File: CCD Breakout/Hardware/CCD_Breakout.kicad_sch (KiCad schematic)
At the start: 6 parts, among them U1 ILX511

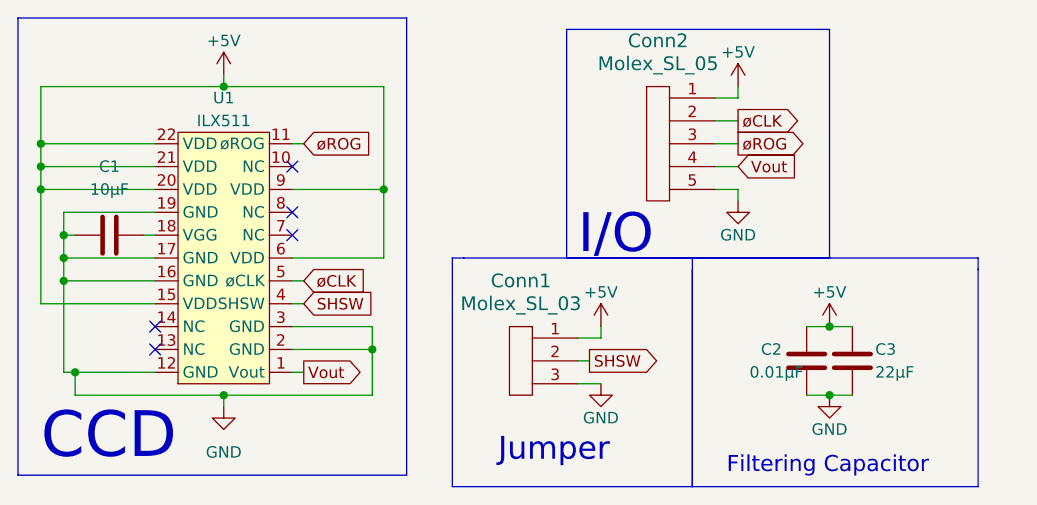
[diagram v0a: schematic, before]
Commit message: misc schematic review changes
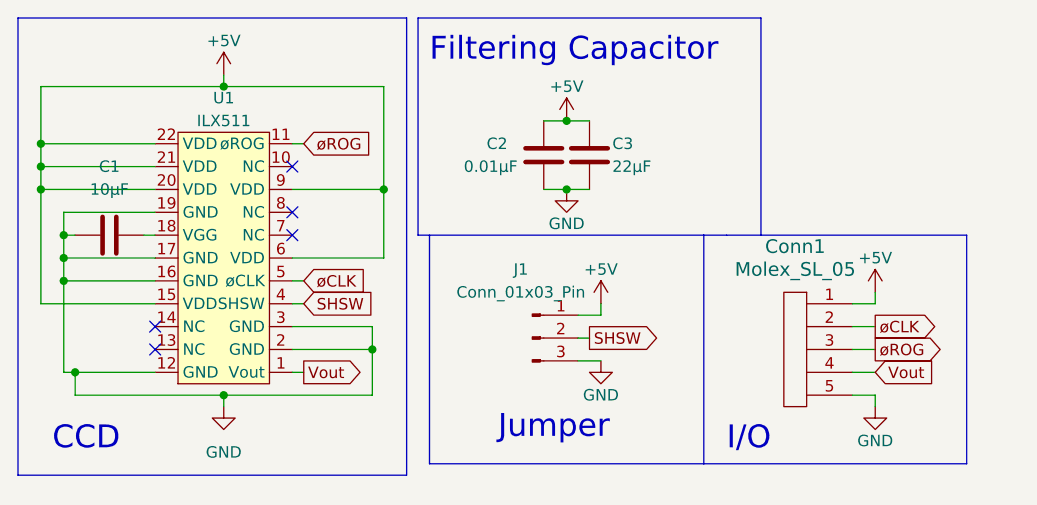
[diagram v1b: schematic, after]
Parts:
- removed Conn1: Molex_SL_03, symbol MRDT_Connectors:Molex_SL_03
- added J1: Conn_01x03_Pin, symbol Connector:Conn_01x03_Pin
- renumbered Conn2 to Conn1
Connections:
- net +5V: now also J1.1 (Pin_1)
- net GND: now also J1.3 (Pin_3)
- net SHSW: now also J1.2 (Pin_2)
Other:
- moved on the sheet: C2, C3, Conn1
